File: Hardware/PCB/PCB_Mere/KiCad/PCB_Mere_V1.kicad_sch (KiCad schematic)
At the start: 24 parts, among them U1 STM32H723ZGTx, U2 SX1276

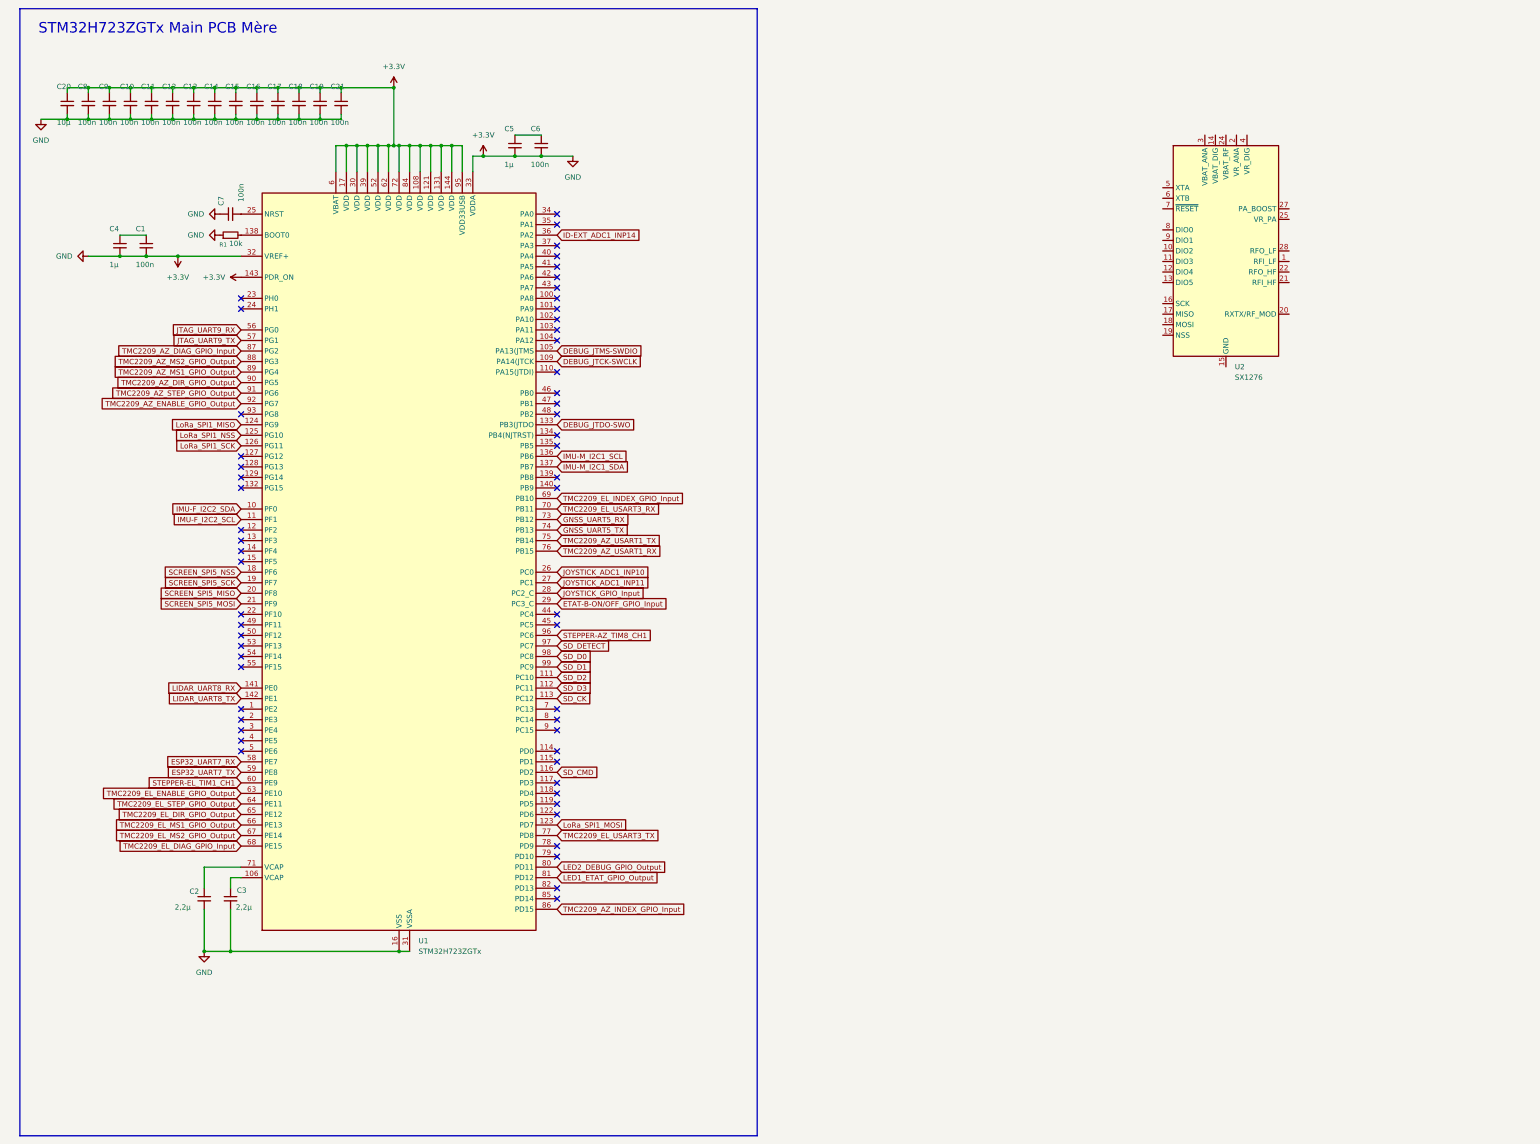
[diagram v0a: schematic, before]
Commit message: Add files via upload
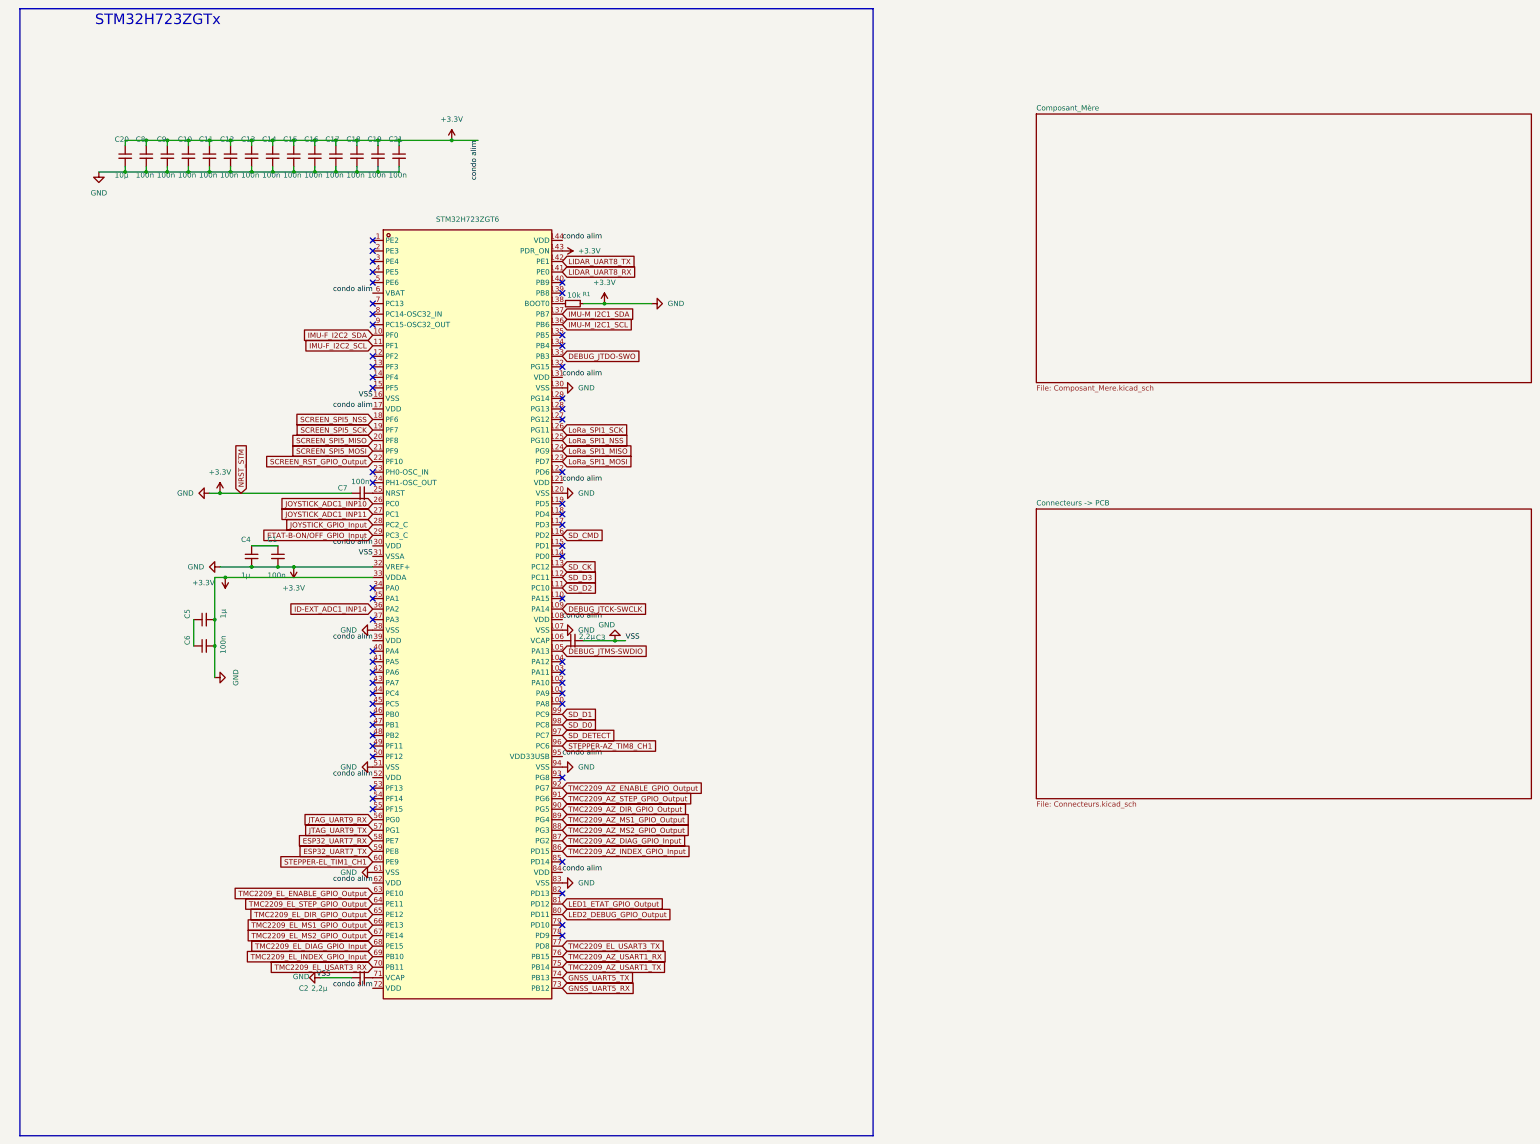
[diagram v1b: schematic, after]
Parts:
- removed U1: STM32H723ZGTx, Package_QFP:LQFP-144_20x20mm_P0.5mm, symbol MCU_ST_STM32H7:STM32H723ZGTx
- removed U2: SX1276, Package_DFN_QFN:QFN-28-1EP_6x6mm_P0.65mm_EP4.8x4.8mm, symbol RF:SX1276
- added U1: STM32H723ZGT6, EasyEDA:LQFP-144_L20.0-W20.0-P0.50-LS22.0-BL, symbol EasyEDA:STM32H723ZGT6
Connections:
- net +3.3V: now also C2.1, U1.107 (VSS), U1.108 (VDD), U1.120 (VSS), U1.121 (VDD), U1.130 (VSS), U1.131 (VDD), U1.143 (PDR_ON), U1.144 (VDD), U1.16 (VSS), U1.17 (VDD), U1.30 (VDD), U1.31 (VSSA), U1.32 (VREF+), U1.33 (VDDA), U1.38 (VSS), U1.39 (VDD), U1.51 (VSS), U1.52 (VDD), U1.6 (VBAT), U1.61 (VSS), U1.62 (VDD), U1.72 (VDD), U1.83 (VSS), U1.84 (VDD), U1.94 (VSS), U1.95 (VDD33USB); no longer C2.2
- net DEBUG_JTCK-SWCLK: now also U1.109 (PA14)
- net DEBUG_JTDO-SWO: now also U1.133 (PB3)
- net DEBUG_JTMS-SWDIO: now also U1.105 (PA13)
- net ESP32_UART7_RX: now also U1.58 (PE7)
- net ESP32_UART7_TX: now also U1.59 (PE8)
- net ETAT-B-ON/OFF_GPIO_Input: now also U1.29 (PC3_C)
- net GNSS_UART5_RX: now also U1.73 (PB12)
- net GNSS_UART5_TX: now also U1.74 (PB13)
- net ID-EXT_ADC1_INP14: now also U1.36 (PA2)
- net IMU-F_I2C2_SCL: now also U1.11 (PF1)
- net IMU-F_I2C2_SDA: now also U1.10 (PF0)
- net IMU-M_I2C1_SCL: now also U1.136 (PB6)
- net IMU-M_I2C1_SDA: now also U1.137 (PB7)
- net JOYSTICK_ADC1_INP10: now also U1.26 (PC0)
- net JOYSTICK_ADC1_INP11: now also U1.27 (PC1)
- net JOYSTICK_GPIO_Input: now also U1.28 (PC2_C)
- net JTAG_UART9_RX: now also U1.56 (PG0)
- net JTAG_UART9_TX: now also U1.57 (PG1)
- net LED1_ETAT_GPIO_Output: now also U1.81 (PD12)
- net LED2_DEBUG_GPIO_Output: now also U1.80 (PD11)
- net LIDAR_UART8_RX: now also U1.141 (PE0)
- net LIDAR_UART8_TX: now also U1.142 (PE1)
- net LoRa_SPI1_MISO: now also U1.124 (PG9)
- net LoRa_SPI1_MOSI: now also U1.123 (PD7)
- net LoRa_SPI1_NSS: now also U1.125 (PG10)
- net LoRa_SPI1_SCK: now also U1.126 (PG11)
- net SCREEN_SPI5_MISO: now also U1.20 (PF8)
- net SCREEN_SPI5_MOSI: now also U1.21 (PF9)
- net SCREEN_SPI5_NSS: now also U1.18 (PF6)
- net SCREEN_SPI5_SCK: now also U1.19 (PF7)
- net SD_CK: now also U1.113 (PC12)
- net SD_CMD: now also U1.116 (PD2)
- net SD_D0: now also U1.98 (PC8)
- net SD_D1: now also U1.99 (PC9)
- net SD_D2: now also U1.111 (PC10)
- net SD_D3: now also U1.112 (PC11)
- net SD_DETECT: now also U1.97 (PC7)
- net STEPPER-AZ_TIM8_CH1: now also U1.96 (PC6)
- net STEPPER-EL_TIM1_CH1: now also U1.60 (PE9)
- net TMC2209_AZ_DIAG_GPIO_Input: now also U1.87 (PG2)
- net TMC2209_AZ_DIR_GPIO_Output: now also U1.90 (PG5)
- net TMC2209_AZ_ENABLE_GPIO_Output: now also U1.92 (PG7)
- net TMC2209_AZ_INDEX_GPIO_Input: now also U1.86 (PD15)
- net TMC2209_AZ_MS1_GPIO_Output: now also U1.89 (PG4)
- net TMC2209_AZ_MS2_GPIO_Output: now also U1.88 (PG3)
- net TMC2209_AZ_STEP_GPIO_Output: now also U1.91 (PG6)
- net TMC2209_AZ_USART1_RX: now also U1.76 (PB15)
- net TMC2209_AZ_USART1_TX: now also U1.75 (PB14)
- net TMC2209_EL_DIAG_GPIO_Input: now also U1.68 (PE15)
- net TMC2209_EL_DIR_GPIO_Output: now also U1.65 (PE12)
- net TMC2209_EL_ENABLE_GPIO_Output: now also U1.63 (PE10)
- net TMC2209_EL_INDEX_GPIO_Input: now also U1.69 (PB10)
- net TMC2209_EL_MS1_GPIO_Output: now also U1.66 (PE13)
- net TMC2209_EL_MS2_GPIO_Output: now also U1.67 (PE14)
- net TMC2209_EL_STEP_GPIO_Output: now also U1.64 (PE11)
- net TMC2209_EL_USART3_RX: now also U1.70 (PB11)
- net TMC2209_EL_USART3_TX: now also U1.77 (PD8)
- net at C7.2: now also U1.25 (NRST)
- net at R1.2: now also U1.138 (BOOT0)
- net at C3.1: now also U1.106 (VCAP)
- new net: C2.2, U1.71 (VCAP)
- new net SCREEN_RST_GPIO_Output: U1.22 (PF10)
- no-connect marks 57 -> 56
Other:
- added sheet Composant_Mère (Composant_Mere.kicad_sch)
- added sheet Connecteurs -> PCB (Connecteurs.kicad_sch)
- note added: "STM32H723ZGTx"
- note removed: "STM32H723ZGTx Main PCB Mère"
- moved on the sheet: C1, C10, C11, C12, C13, C14, C15, C16, C17, C18, C19, C2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
